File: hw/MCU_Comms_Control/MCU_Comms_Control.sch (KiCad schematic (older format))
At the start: 32 parts, among them J1 USB_B_Mini, J2 CAN BUS, J3 TO_POWER_BOARD, J4 Mini-Debugging, J5 MULTI, SW1 BOOT, SW2 BUTTON, U1 SRV05-4, U2 SN65HVD230, U3 W25Q128JVS, U4 STM32F303CCTx, U5 EL817, Y1 12MHz

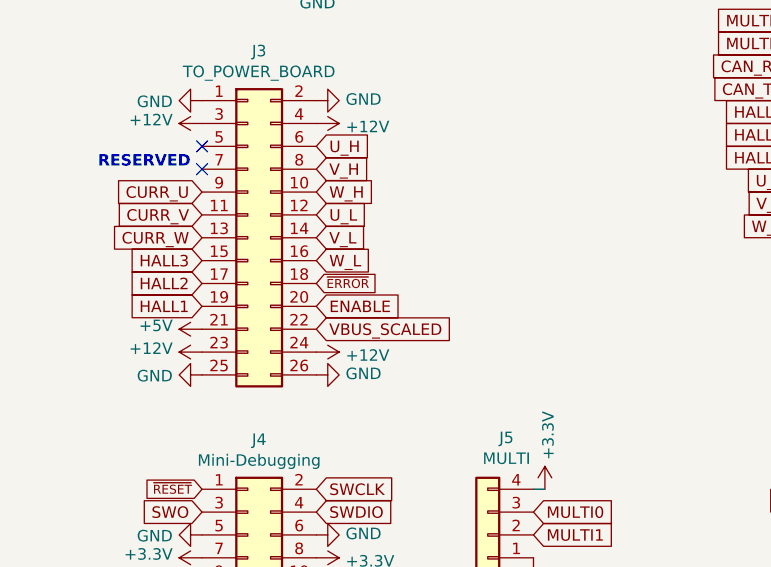
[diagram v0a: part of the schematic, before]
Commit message: advances were made on power electronics board
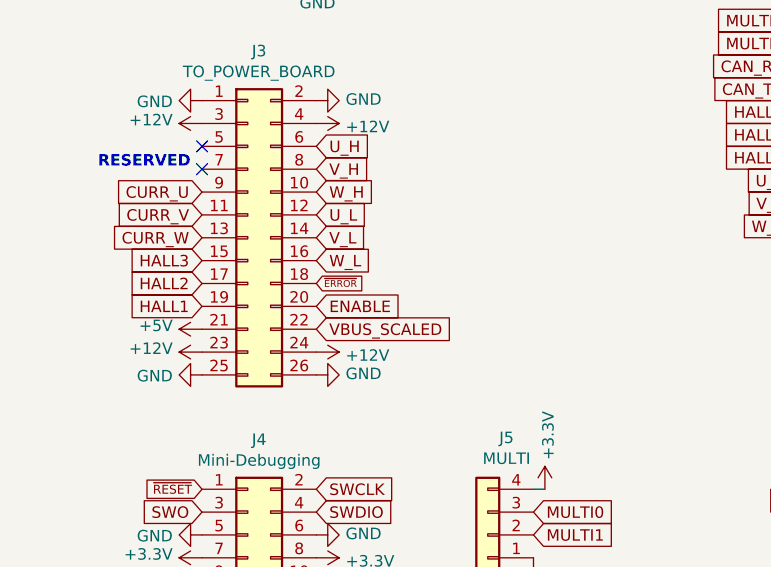
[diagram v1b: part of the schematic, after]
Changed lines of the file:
@@
 	0    -1   -1   0
 $EndComp
-Text GLabel 2000 4300 2    39   Input ~ 0
+Text GLabel 2000 4300 2    30   Input ~ 0
 ~ERROR
 $Comp

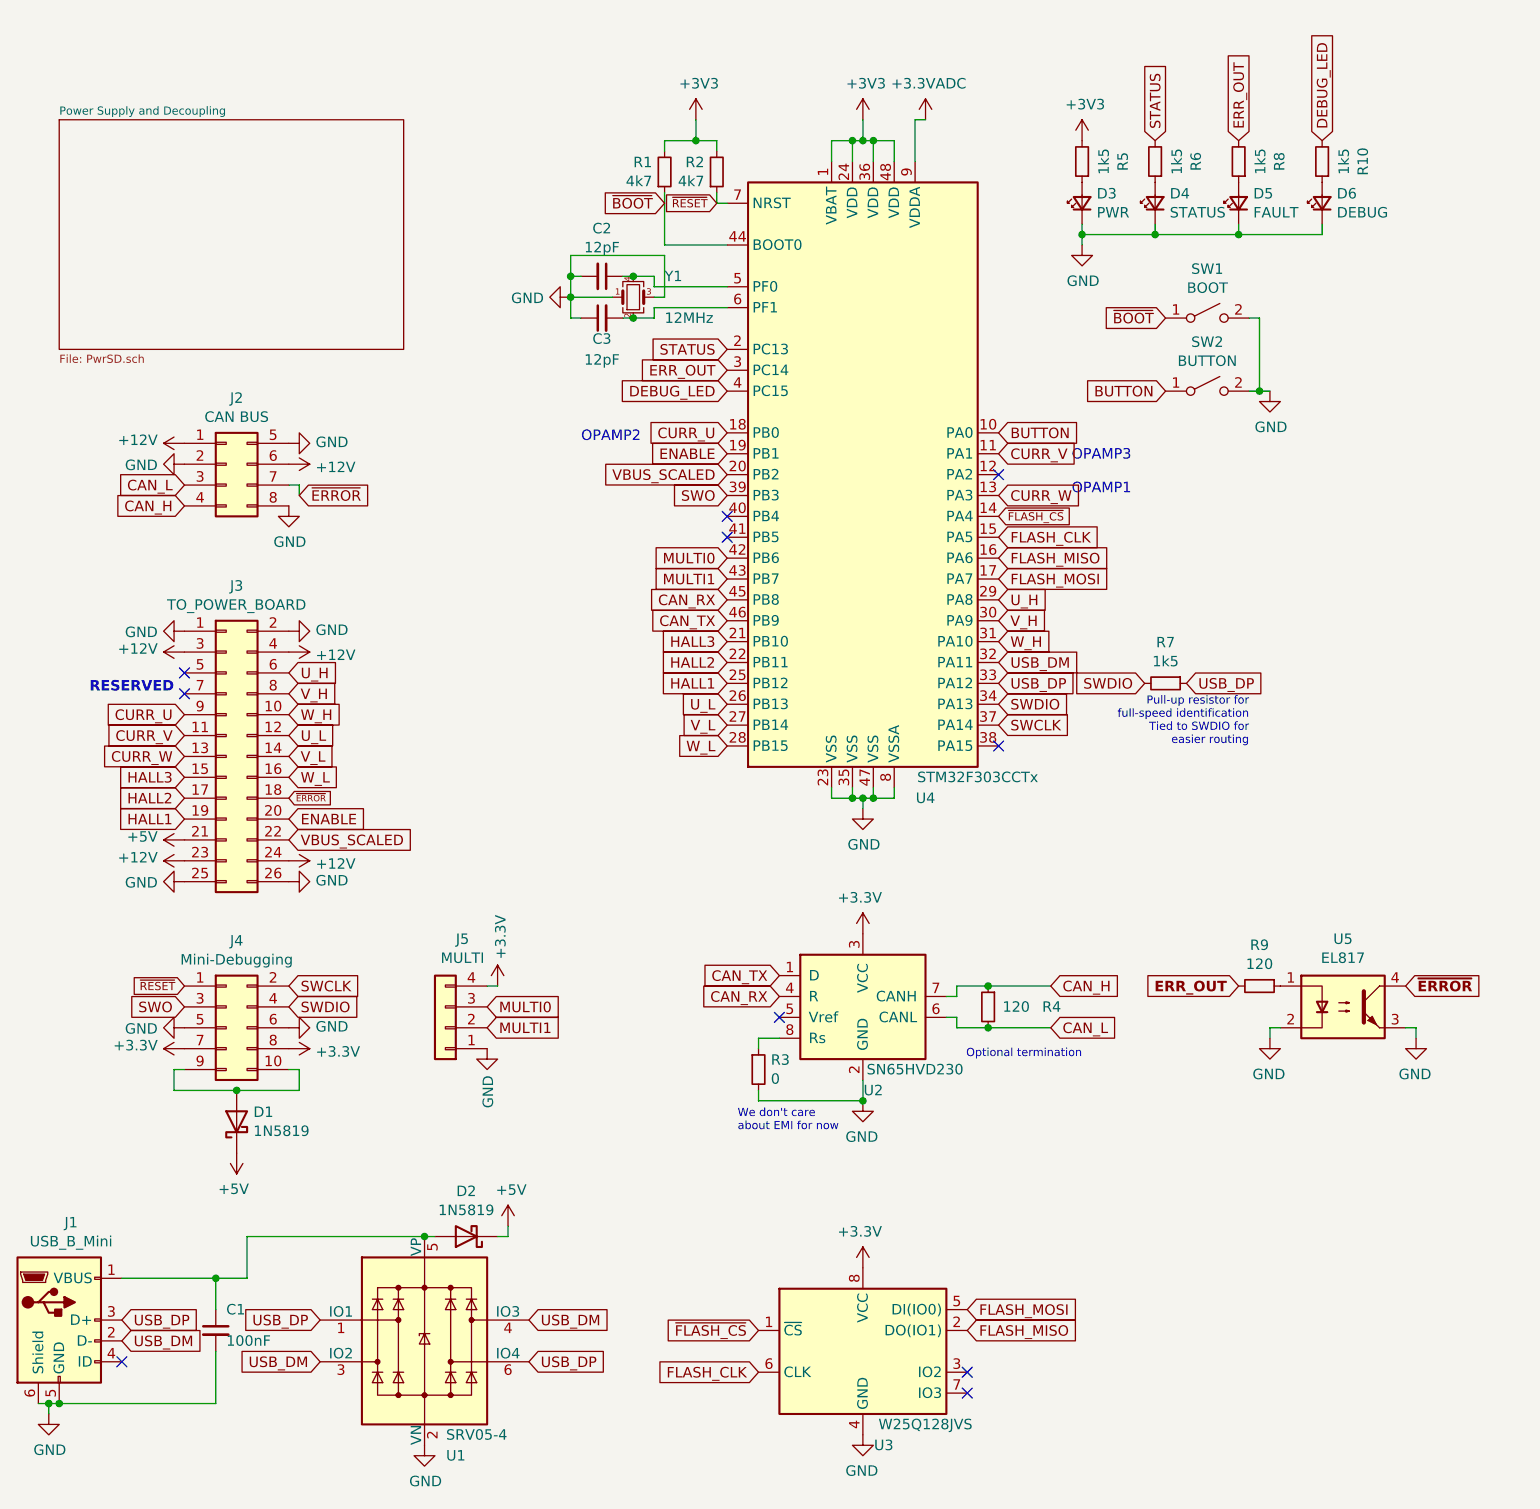
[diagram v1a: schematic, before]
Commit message: remove old gerbers and assembly files
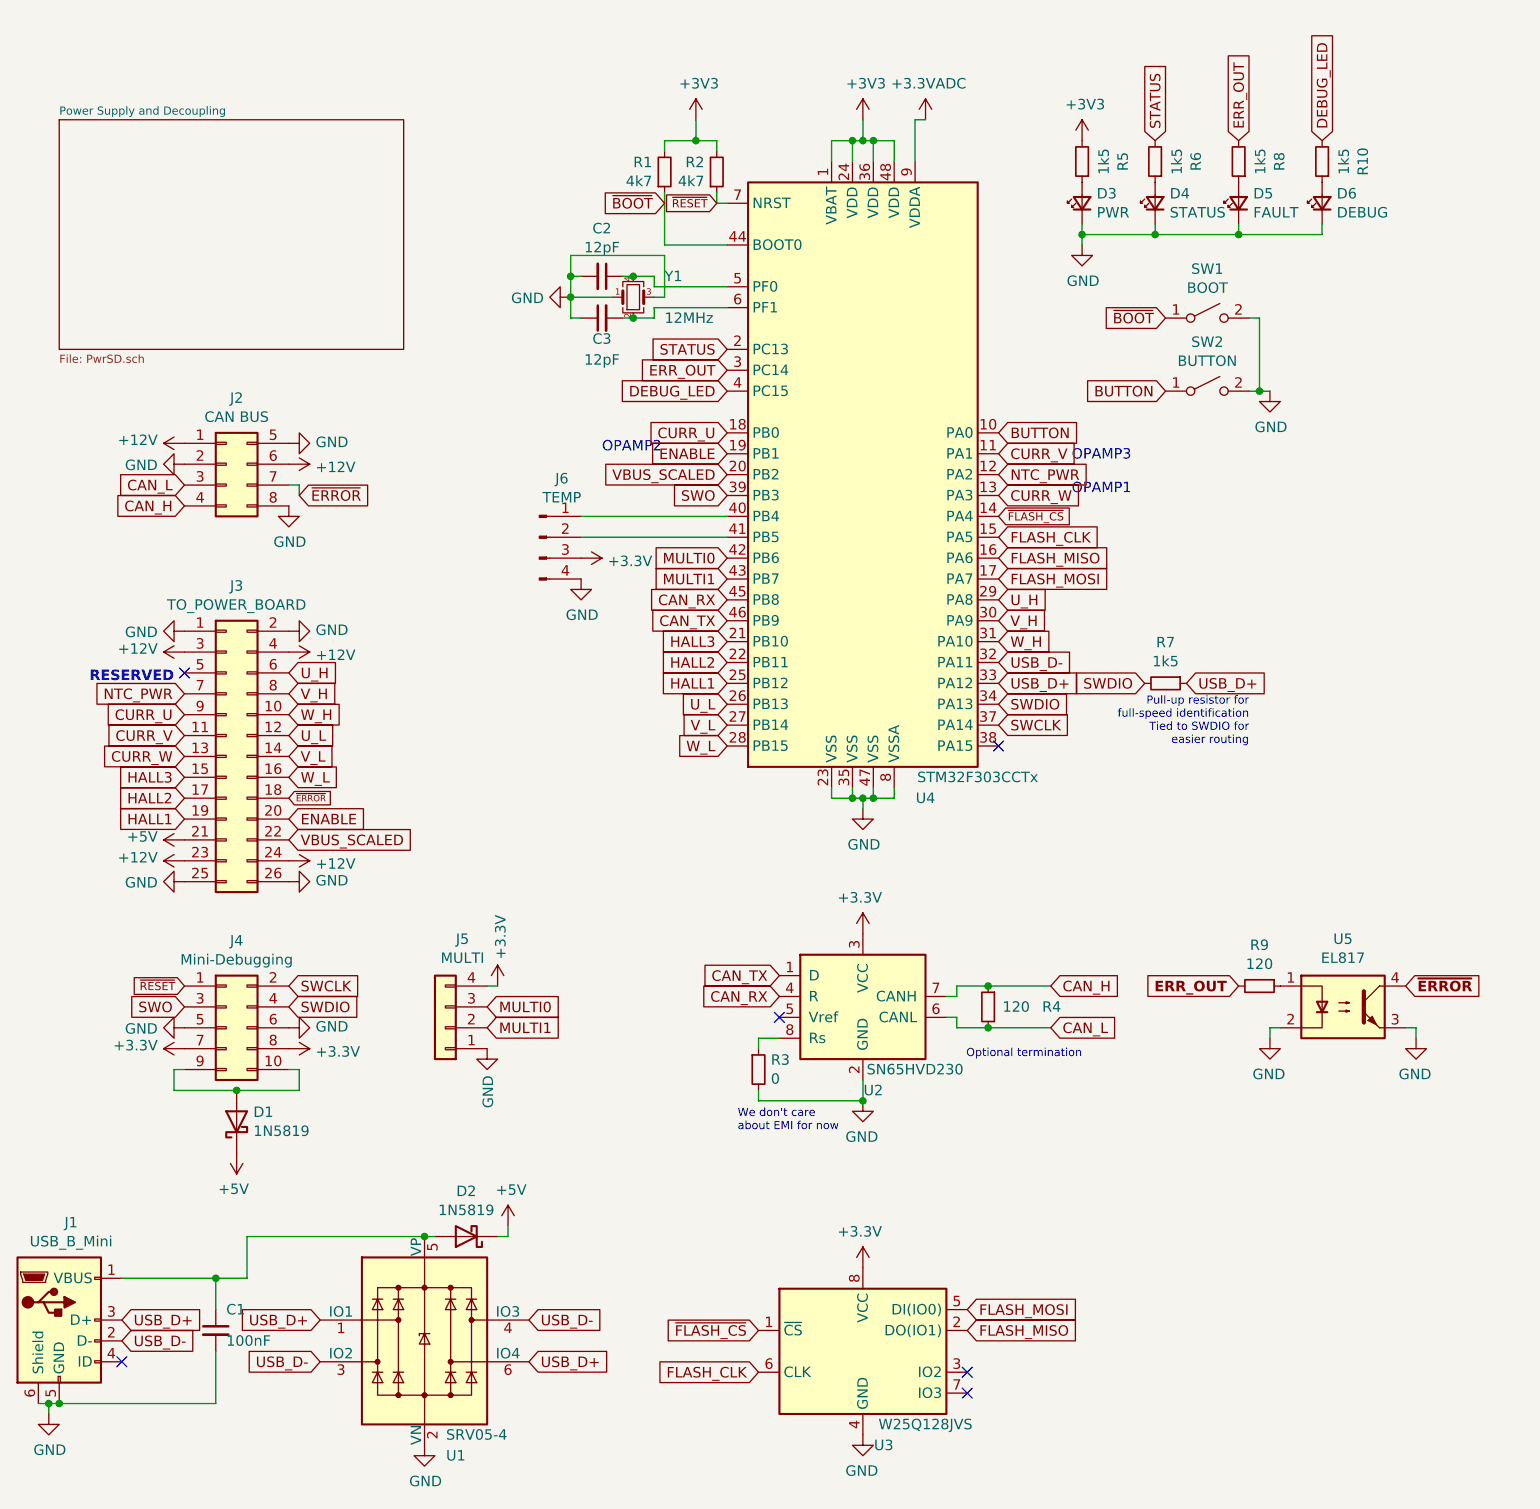
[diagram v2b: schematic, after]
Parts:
- added J6: TEMP, Connector_PinHeader_2.54mm:PinHeader_2x02_P2.54mm_Vertical, symbol Connector:Conn_01x04_Male
- J1: footprint Connector_USB:USB_Micro-B_Molex-105017-0001 -> Connector_USB:USB_Micro-B_Molex-105133-0001
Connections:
- net +3V3: now also J6.3 (Pin_3)
- net GND: now also J6.4 (Pin_4)
- net NTC_PWR: now reaches U4.12 (PA2)
- net NTC_PWR: now also J3.7 (Pin_7)
- net at U4.40 (PB4): now also J6.1 (Pin_1)
- net at U4.41 (PB5): now also J6.2 (Pin_2)
- net USB_DM renamed USB_D-
- net USB_DP renamed USB_D+
- no-connect marks 10 -> 6
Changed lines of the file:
@@
 $EndDescr
-$Comp
-L MCU_ST_STM32F3:STM32F303CCTx U4
-U 1 1 5FB1FDE5
-P 4800 2750
-F 0 "U4" H 5050 1200 50  0000 C CNN
-F 1 "STM32F303CCTx" H 5300 1300 50  0000 C CNN
-F 2 "Package_QFP:LQFP-48_7x7mm_P0.5mm" H 4200 1350 50  0001 R CNN
-F 3 "http://www.st.com/st-web-ui/static/active/en/resource/technical/document/datasheet/DM00058181.pdf" H 4800 2750 50  0001 C CNN
-F 4 "C81523" H 4800 2750 50  0001 C CNN "LCSC"
-	1    4800 2750
-	1    0    0    -1
-$EndComp
 $Comp
 L power:+3V3 #PWR0101
@@
 CAN_TX
 Text GLabel 5400 3750 2    50   Input ~ 0
-USB_DP
+USB_D+
 Text GLabel 5400 3650 2    50   Input ~ 0
-USB_DM
+USB_D-
 $Comp
 L Device:R_Small R7
@@
 $EndComp
 Text GLabel 6300 3750 2    50   Input ~ 0
-USB_DP
+USB_D+
 Text GLabel 6100 3750 0    50   Input ~ 0
 SWDIO
@@
 F 0 "J1" H 957 7267 50  0000 C CNN
 F 1 "USB_B_Mini" H 957 7176 50  0000 C CNN
-F 2 "Connector_USB:USB_Micro-B_Molex-105017-0001" H 1050 6750 50  0001 C CNN
+F 2 "Connector_USB:USB_Micro-B_Molex-105133-0001" H 1050 6750 50  0001 C CNN
 F 3 "~" H 1050 6750 50  0001 C CNN
 	1    900  6800
@@
 HALL3
 NoConn ~ 1500 3700
-NoConn ~ 1500 3800
-Text Notes 1450 3800 2    50   ~ 10
+Text Notes 1450 3750 2    50   ~ 10
 RESERVED
 $Comp
@@
 $EndComp
 Text GLabel 1200 6900 2    50   Input ~ 0
-USB_DM
+USB_D-
 Text GLabel 1200 6800 2    50   Input ~ 0
-USB_DP
+USB_D+
 Text GLabel 2150 6800 0    50   Input ~ 0
-USB_DP
+USB_D+
 Text GLabel 2150 7000 0    50   Input ~ 0
-USB_DM
+USB_D-
 Wire Wire Line
 	2650 6400 1800 6400
@@
 Text Notes 5750 2850 0    50   ~ 0
 OPAMP3\n\nOPAMP1
-Text Notes 3400 2600 0    50   ~ 0
+Text Notes 3500 2650 0    50   ~ 0
 OPAMP2\n
 Text GLabel 4100 2750 0    50   Input ~ 0
@@
 Text GLabel 5400 2550 2    50   Input ~ 0
 BUTTON
-NoConn ~ 5400 2750
-NoConn ~ 4100 2950
-NoConn ~ 4100 3050
 NoConn ~ 1200 7000
 NoConn ~ 5250 7050
@@
 Connection ~ 3350 1800
 Text GLabel 3150 7000 2    50   Input ~ 0
-USB_DP
+USB_D+
 Text GLabel 3150 6800 2    50   Input ~ 0
-USB_DM
+USB_D-
 $Comp
 L Connector_Generic:Conn_02x13_Odd_Even J3
@@
 $EndComp
 NoConn ~ 5400 4050
+$Comp
+L MCU_ST_STM32F3:STM32F303CCTx U4
+U 1 1 5FB1FDE5
+P 4800 2750
+F 0 "U4" H 5050 1200 50  0000 C CNN
+F 1 "STM32F303CCTx" H 5300 1300 50  0000 C CNN
+F 2 "Package_QFP:LQFP-48_7x7mm_P0.5mm" H 4200 1350 50  0001 R CNN
+F 3 "http://www.st.com/st-web-ui/static/active/en/resource/technical/document/datasheet/DM00058181.pdf" H 4800 2750 50  0001 C CNN
+F 4 "C81523" H 4800 2750 50  0001 C CNN "LCSC"
+	1    4800 2750
+	1    0    0    -1
+$EndComp
+$Comp
+L power:GND #PWR01
+U 1 1 5FD220C9
+P 3400 3250
+F 0 "#PWR01" H 3400 3000 50  0001 C CNN
+F 1 "GND" H 3405 3077 50  0000 C CNN
+F 2 "" H 3400 3250 50  0001 C CNN
+F 3 "" H 3400 3250 50  0001 C CNN
+	1    3400 3250
+	1    0    0    -1
+$EndComp
+$Comp
+L Connector:Conn_01x04_Male J6
+U 1 1 5FD31C82
+P 3200 3050
+F 0 "J6" H 3308 3331 50  0000 C CNN
+F 1 "TEMP" H 3308 3240 50  0000 C CNN
+F 2 "Connector_PinHeader_2.54mm:PinHeader_2x02_P2.54mm_Vertical" H 3200 3050 50  0001 C CNN
+F 3 "~" H 3200 3050 50  0001 C CNN
+	1    3200 3050
+	1    0    0    -1
+$EndComp
+$Comp
+L power:+3.3V #PWR02
+U 1 1 5FD36362
+P 3400 3150
+F 0 "#PWR02" H 3400 3000 50  0001 C CNN
+F 1 "+3.3V" V 3415 3278 50  0000 L CNN
+F 2 "" H 3400 3150 50  0001 C CNN
+F 3 "" H 3400 3150 50  0001 C CNN
+	1    3400 3150
+	0    1    1    0
+$EndComp
+Wire Wire Line
+	3400 3050 4100 3050
+Wire Wire Line
+	4100 2950 3400 2950
+Text GLabel 1500 3800 0    50   Input ~ 0
+NTC_PWR
+Text GLabel 5400 2750 2    50   Input ~ 0
+NTC_PWR
 $EndSCHEMATC
